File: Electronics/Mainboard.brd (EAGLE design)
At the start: 100 x 80 mm, 37 parts, among them IC1 4081N, IC2 4069N, Q1 IRFZ48V, Q2 IRF4905V, Q3 IRFZ48V, Q4 IRF4905V, Q5 IRFZ48V, Q6 IRF4905V, Q7 IRFZ48V, Q8 IRF4905V, X3 24V Batt

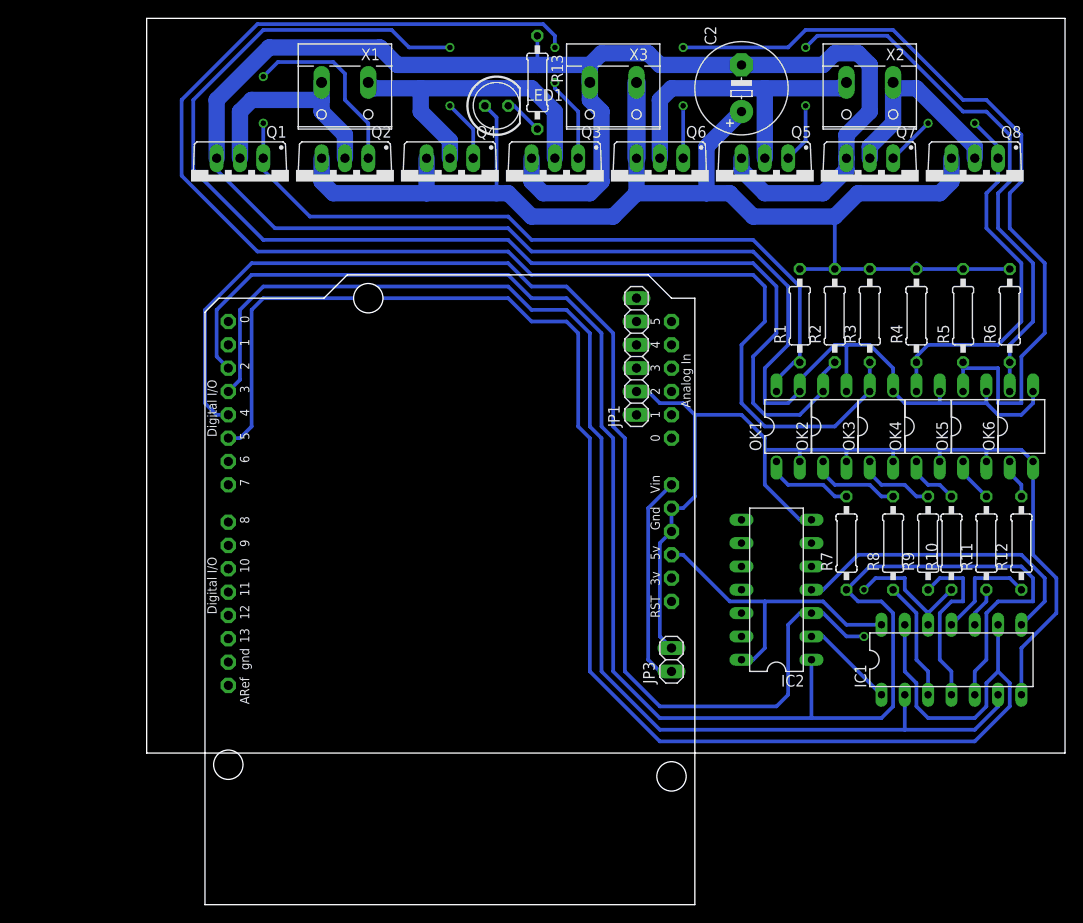
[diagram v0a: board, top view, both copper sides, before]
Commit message: 
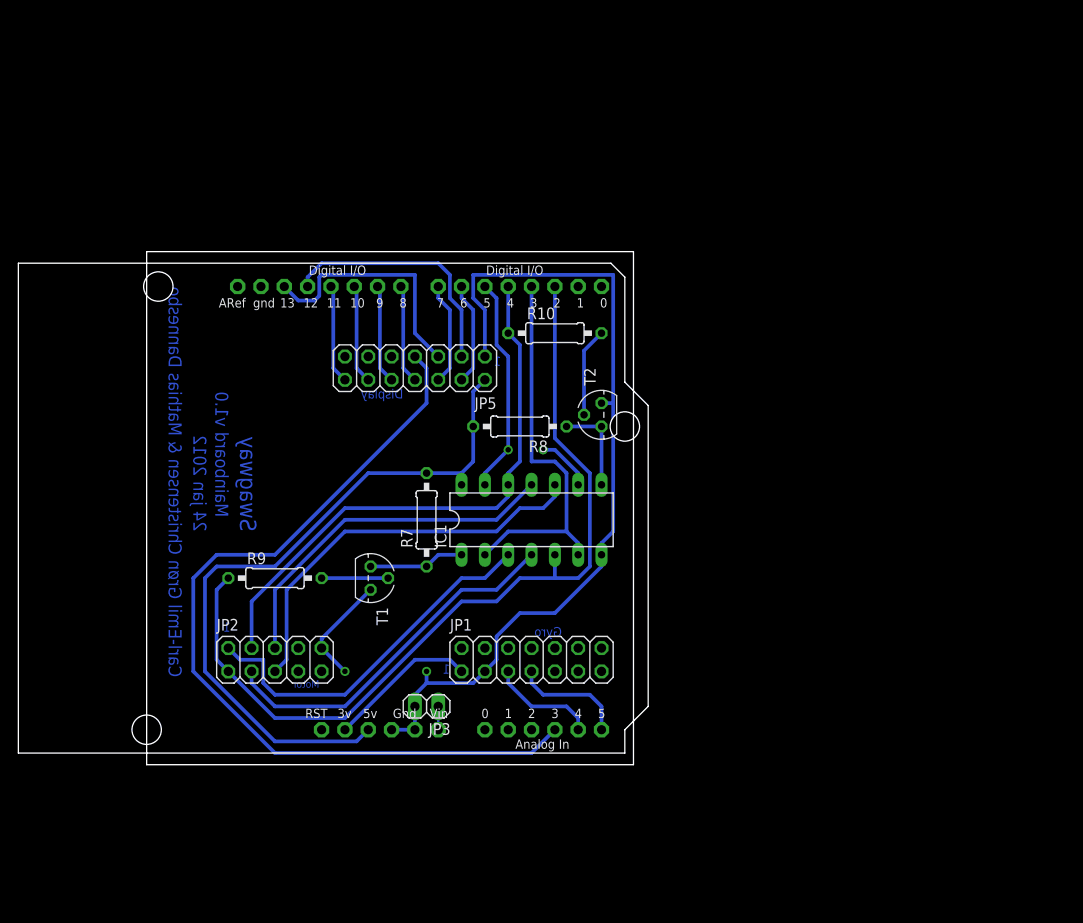
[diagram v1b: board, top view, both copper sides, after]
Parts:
- removed C2: (no value), rcl:E5-10,5
- removed IC2: 4069N, 40xx:DIL14
- removed LED1: (no value), led:LED5MM
- removed OK1, OK2, OK3, OK4, OK5, OK6: PC817, optocoupler:DIL04
- removed Q1, Q3, Q5, Q7: IRFZ48V, transistor-power:TO220BV
- removed Q2, Q4, Q6, Q8: IRF4905V, transistor-power:TO220BV
- removed R1, R2, R3, R4, R5, R6: 10k, rcl:0207/10
- removed R11, R12: 180, rcl:0207/10
- removed R13: 1k, rcl:0207/10
- removed X1, X2: (no value), con-wago-508:W237-132
- removed X3: 24V Batt, con-wago-508:W237-132
- added JP2: Motorcontroller, pinhead:2X05
- added JP5: Display, pinhead:2X07
- added T1, T2: BC547, transistor:TO92
- JP1: device pinhead:1X06 -> pinhead:2X07
- R10, R9: value 180 -> 1k
- R7, R8: value 180 -> 10k
- moved U$1 75.5 mm to (-14.0, 0.00), turned to 0 degrees
- moved R9 71.2 mm to (14.0, 19.1), turned to 0 degrees
- moved R10 48.9 mm to (44.5, 45.7), turned to 0 degrees
- moved IC1 48.2 mm to (41.9, 25.4)
- moved R7 45.8 mm to (30.5, 25.4)
- moved R8 42.6 mm to (40.6, 35.6), turned to 180 degrees
- moved JP1 34.9 mm to (41.9, 10.2), turned to 0 degrees
- moved JP3 27.1 mm to (30.5, 5.08), turned to 180 degrees
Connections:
- removed net +24V: C2.+, LED1.A, Q2.S, Q4.S, Q6.S, Q8.S, R1.2, R2.2, R3.2, R4.2, R5.2, R6.2, X3.1
- removed net GND2: C2.-, OK1.3, OK2.3, OK3.3, OK4.3, OK5.3, OK6.3, Q1.S, Q3.S, Q5.S, Q7.S, R13.1, X3.2
- removed net N$12: OK1.4, Q1.G, Q2.G, R1.1
- removed net N$13: OK3.4, Q3.G, R3.1
- removed net N$14: OK3.1, R9.2
- removed net N$15: IC1.3, R8.1
- removed net N$18: Q7.D, Q8.D, X2.1
- removed net N$19: OK4.4, Q7.G, Q8.G, R4.1
- removed net N$21: OK5.4, Q6.G, R5.1
- removed net N$22: OK6.4, Q5.G, R6.1
- removed net N$23: OK6.1, R12.2
- removed net N$24: IC1.10, R11.1
- removed net N$25: IC1.11, R12.1
- removed net N$27: IC1.12, IC2.3, R10.1, U$1.D4
- removed net N$28: OK1.1, R7.2
- removed net N$6: LED1.K, R13.2
- removed net N$9: OK2.4, Q4.G, R2.1
- removed net VCC: IC1.14, IC2.14, U$1.5V
- new net +5V: IC1.14, JP5.2, R7.2, R8.2, U$1.5V
- new net N$31: JP5.4, U$1.D6
- new net N$38: JP5.8, U$1.D8
- new net N$40: JP5.10, U$1.D9
- new net N$43: JP5.14, U$1.D11
- new net N$44: JP5.3, U$1.D12
- new net N$45: JP5.5, U$1.D13
- new net N$46: JP5.7, U$1.A3
- net GND: now also JP1.3, JP2.10, JP5.1, T1.1, T2.1; no longer IC2.7, JP1.2, OK1.2, OK2.2, OK3.2, OK4.2, OK5.2, OK6.2
- net N$1: now also IC1.3, JP2.2; no longer Q5.D, Q6.D, X2.2
- net N$10: now also JP2.1, R9.1; no longer IC2.1, R7.1
- net N$16: now also R8.1, T2.3; no longer IC2.4
- net N$17: now also R9.2, T1.2; no longer IC1.4, R9.1
- net N$2: now also IC1.4, JP2.3; no longer Q3.D, Q4.D, X1.1
- net N$20: now also R10.2, T2.2; no longer OK5.1, R11.2
- net N$26: now also JP1.7
- net N$3: now also IC1.12, JP2.4, R10.1, U$1.D4; no longer OK2.1, R8.2
- net N$37: now also JP5.6, U$1.D7; no longer U$1.A4
- net N$4: now also IC1.10, JP2.5; no longer Q1.D, Q2.D, X1.2
- net N$41: now also JP1.5, U$1.A4; no longer JP1.3
- net N$42: now also JP5.12, U$1.D10; no longer JP1.4
- net N$5: now also IC1.11, JP2.6; no longer OK4.1, R10.2
- net N$8: now also R7.1, T1.3; no longer IC2.2
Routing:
- net GND2: track 267.4 -> 0.00 mm
- net N$13: track 165.4 -> 0.00 mm, vias 1 -> 0
- net N$27: track 152.3 -> 0.00 mm
- net +24V: track 144.2 -> 0.00 mm
- net N$7: track 173.1 -> 29.8 mm, vias 0 -> 1
- net N$9: track 141.7 -> 0.00 mm, vias 2 -> 1
- net N$12: track 101.9 -> 0.00 mm, vias 2 -> 1
- net N$11: track 141.2 -> 42.7 mm
- net N$21: track 93.8 -> 0.00 mm, vias 1 -> 0
- net N$46: track 0.00 -> 93.2 mm
- net N$10: track 185.6 -> 94.1 mm
- net +5V: track 0.00 -> 76.8 mm
- net N$22: track 64.8 -> 0.00 mm
- net N$3: track 9.94 -> 61.7 mm
- net N$19: track 47.0 -> 0.00 mm, vias 2 -> 0
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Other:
- board size 100 x 80 mm -> 68.6 x 53.3 mm
- board text added: "1"
- board text added: "24 jan 2012"
- board text added: "Carl-Emil Grøn Christensen & Mathias Dannesbo"
- board text added: "Display"
- board text added: "Gyro"
- board text added: "Mainboard v1.0"
- board text added: "Motor"
- board text added: "Swagway"
